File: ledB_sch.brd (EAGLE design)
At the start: 22.9 x 22.9 mm, 7 parts

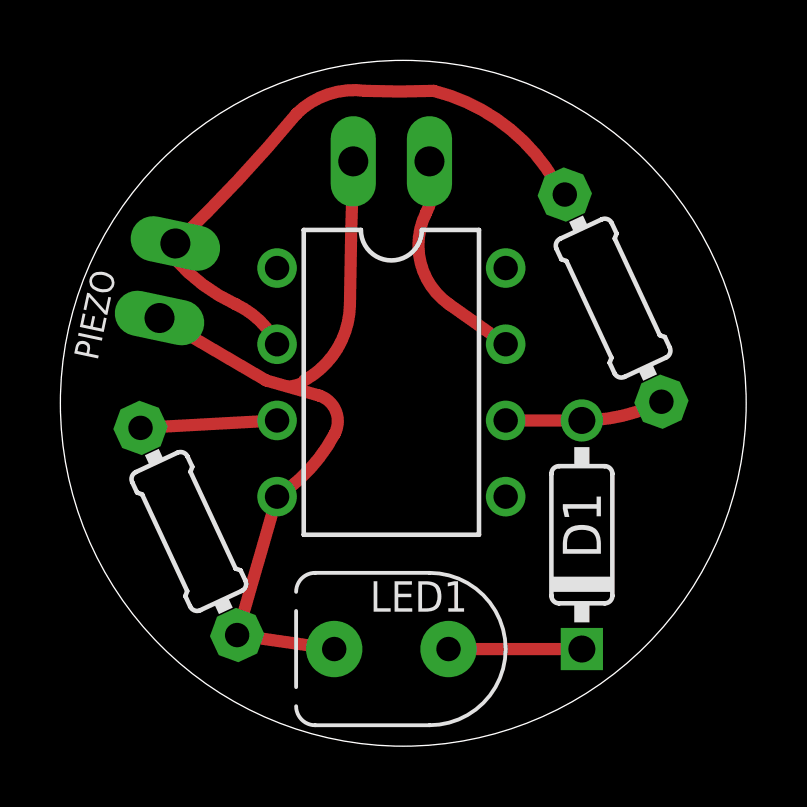
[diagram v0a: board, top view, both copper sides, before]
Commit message: smd
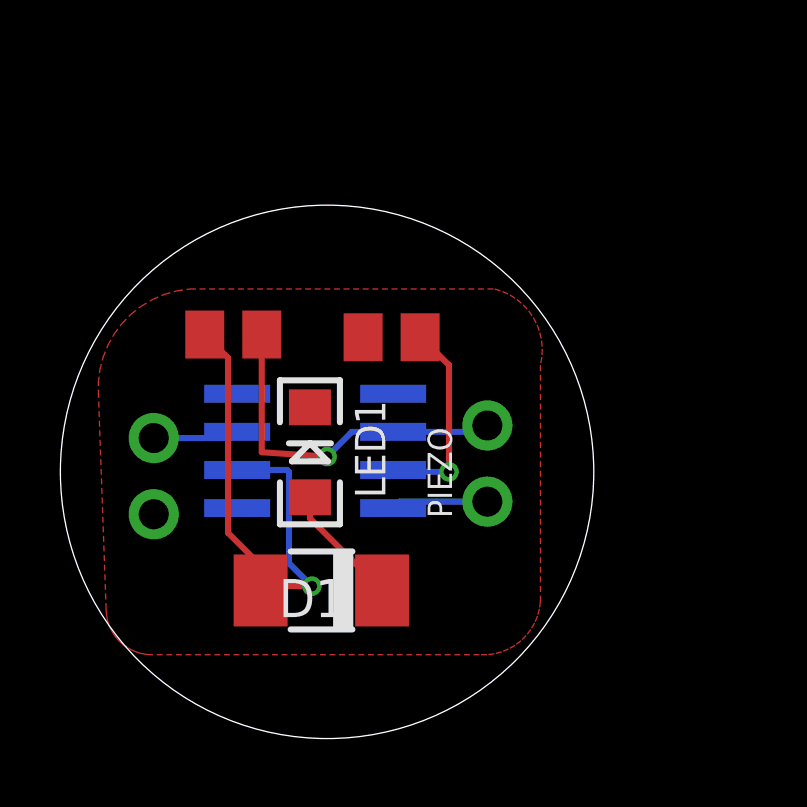
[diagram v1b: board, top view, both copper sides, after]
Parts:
- D1: value diode -> 1N4001; device ledB_sch:DO35-3 -> diode:DO-214AC
- JP1: device ledB_sch:1X02_OVAL -> ledB_sch:1X02_ROUND
- LED1: device ledB_sch:LED5MM -> ledB_sch:LED-1206
- OPAMP: device ledB_sch:DIL08 -> ledB_sch:SO08
- PIEZO: device ledB_sch:1X02_PEIZO -> ledB_sch:1X02_ROUND
- R1, R2: device ledB_sch:0204/7 -> ledB_sch:M0805
- moved JP1 13.1 mm to (3.11, 9.00), turned to 90 degrees
- moved R2 12.7 mm to (5.76, 13.7), turned to 0 degrees
- moved PIEZO 12.3 mm to (14.2, 9.42), turned to 90 degrees
- moved R1 9.36 mm to (11.0, 13.6), turned to 0 degrees
- moved D1 8.88 mm to (8.70, 5.19), turned to 180 degrees
- moved LED1 7.10 mm to (8.32, 9.79), turned to 90 degrees
- moved OPAMP 3.42 mm to (8.49, 9.84), flipped to the bottom
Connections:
- net GND: now also LED1.C; no longer LED1.K
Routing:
- net GND: track 27.2 -> 3.23 mm
- net N$2: track 5.26 -> 16.9 mm, vias 0 -> 1
- net SIG: track 21.3 -> 11.9 mm, vias 0 -> 1
- net VCC: track 7.17 -> 2.87 mm
- net N$1: track 4.56 -> 6.79 mm, vias 0 -> 1
- added copper zone on layer 1, net GND
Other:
- board size 22.9 x 22.9 mm -> 17.8 x 17.8 mm
